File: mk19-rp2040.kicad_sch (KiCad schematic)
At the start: 134 parts, among them J1 USB_C_Receptacle_USB2.0, J10 Conn_01x02, J11 Conn_01x03_Socket, J12 USB_C_Receptacle_USB2.0, J13 USB_C_Receptacle_USB2.0, J3 Conn_01x02_Socket, J5 Conn_01x02, J7 Conn_01x02_Socket, J8 Conn_01x02_Socket, J9 Conn_01x02_Socket, T1 Conn_01x01_Socket, T10 Conn_01x01_Socket, T11 Conn_01x01_Socket, T12 Conn_01x01_Socket, T13 Conn_01x01_Socket, T14 Conn_01x01_Socket, T15 Conn_01x01_Socket, T2 Conn_01x01_Socket, T3 Conn_01x01_Socket, T5 Conn_01x01_Socket, T6 Conn_01x01_Socket, T7 Conn_01x01_Socket, T8 Conn_01x01_Socket, T9 Conn_01x01_Socket, U1 RP2040, U10 1N4148W_C81598, U11 1N4148W_C81598, U12 1N4148W_C81598, U13 1N4148W_C81598, U14 1N4148W_C81598, U15 1N4148W_C81598, U2 USBLC6-2P6, U3 XC6210B332MR-G, U4 USBLC6-2P6, U5 W25Q128JVS, U6 8_01A0_008200, U7 8_01A0_008200, U8 USBLC6-2P6, U9 1N4148W_C81598, Y1 Crystal_GND24

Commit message: some bad footprints, other fixes
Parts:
- 5WAY1, FAL1, FAL2, PWM1: footprint Connector_JST:JST_XH_B3B-XH-AM_1x08_P2.50mm_Horizontal -> Connector_JST:JST_XH_S8B-XH-A_1x08_P2.50mm_Horizontal
- COL1, COL2, ROW1, ROW2: footprint Connector_JST:JST_EH_S8B-EH_1x08_P2.50mm_Horizontal -> Connector_JST:JST_XH_S8B-XH-A_1x08_P2.50mm_Horizontal
- J1, J12, J13: footprint drawings:GT-USB-7014C -> ct-kicad:USB-C-SMD_12P-P0.50-H-F_TYPE-C-31-M-14
- J3, J7, J8, J9, PWR-EXT-IN1: footprint Connector_JST:JST_XH_B3B-XH-AM_1x02_P2.50mm_Vertical -> Connector_JST:JST_XH_B2B-XH-AM_1x02_P2.50mm_Vertical
- VANILED1: footprint Connector_JST:JST_XH_B3B-XH-AM_1x08_P2.50mm_Vertical -> Connector_JST:JST_XH_B8B-XH-AM_1x08_P2.50mm_Vertical
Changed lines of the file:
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@@
 			)
 		)
-		(property "Footprint" "Connector_JST:JST_XH_B3B-XH-AM_1x08_P2.50mm_Horizontal"
+		(property "Footprint" "Connector_JST:JST_XH_S8B-XH-A_1x08_P2.50mm_Horizontal"
 			(at 158.75 271.78 0)
 			(effects
@@
 			)
 		)
-		(property "Footprint" "Connector_JST:JST_XH_B3B-XH-AM_1x08_P2.50mm_Horizontal"
+		(property "Footprint" "Connector_JST:JST_XH_S8B-XH-A_1x08_P2.50mm_Horizontal"
 			(at 100.33 269.24 0)
 			(effects
@@
 			)
 		)
-		(property "Footprint" "drawings:GT-USB-7014C"
+		(property "Footprint" "ct-kicad:USB-C-SMD_12P-P0.50-H-F_TYPE-C-31-M-14"
 			(at 373.38 367.03 0)
 			(effects
@@
 			)
 		)
-		(property "Footprint" "Connector_JST:JST_XH_B3B-XH-AM_1x02_P2.50mm_Vertical"
+		(property "Footprint" "Connector_JST:JST_XH_B2B-XH-AM_1x02_P2.50mm_Vertical"
 			(at 229.87 429.26 0)
 			(effects
@@
 			)
 		)
-		(property "Footprint" "Connector_JST:JST_XH_B3B-XH-AM_1x02_P2.50mm_Vertical"
+		(property "Footprint" "Connector_JST:JST_XH_B2B-XH-AM_1x02_P2.50mm_Vertical"
 			(at 134.62 411.48 0)
 			(effects
@@
 			)
 		)
-		(property "Footprint" "Connector_JST:JST_XH_B3B-XH-AM_1x08_P2.50mm_Horizontal"
+		(property "Footprint" "Connector_JST:JST_XH_S8B-XH-A_1x08_P2.50mm_Horizontal"
 			(at 46.99 269.24 0)
 			(effects
@@
 			)
 		)
-		(property "Footprint" "drawings:GT-USB-7014C"
+		(property "Footprint" "ct-kicad:USB-C-SMD_12P-P0.50-H-F_TYPE-C-31-M-14"
 			(at 374.65 237.49 0)
 			(effects
@@
 			)
 		)
-		(property "Footprint" "Connector_JST:JST_EH_S8B-EH_1x08_P2.50mm_Horizontal"
+		(property "Footprint" "Connector_JST:JST_XH_S8B-XH-A_1x08_P2.50mm_Horizontal"
 			(at 44.45 148.59 0)
 			(effects
@@
 			)
 		)
-		(property "Footprint" "Connector_JST:JST_EH_S8B-EH_1x08_P2.50mm_Horizontal"
+		(property "Footprint" "Connector_JST:JST_XH_S8B-XH-A_1x08_P2.50mm_Horizontal"
 			(at 71.12 148.59 0)
 			(effects
@@
 			)
 		)
-		(property "Footprint" "Connector_JST:JST_XH_B3B-XH-AM_1x02_P2.50mm_Vertical"
+		(property "Footprint" "Connector_JST:JST_XH_B2B-XH-AM_1x02_P2.50mm_Vertical"
 			(at 209.55 403.86 0)
 			(effects
@@
 			)
 		)
-		(property "Footprint" "Connector_JST:JST_EH_S8B-EH_1x08_P2.50mm_Horizontal"
+		(property "Footprint" "Connector_JST:JST_XH_S8B-XH-A_1x08_P2.50mm_Horizontal"
 			(at 71.12 123.19 0)
 			(effects
@@
 			)
 		)
-		(property "Footprint" "Connector_JST:JST_XH_B3B-XH-AM_1x08_P2.50mm_Vertical"
+		(property "Footprint" "Connector_JST:JST_XH_B8B-XH-AM_1x08_P2.50mm_Vertical"
 			(at 166.37 370.84 0)
 			(effects
@@
 			)
 		)
-		(property "Footprint" "drawings:GT-USB-7014C"
+		(property "Footprint" "ct-kicad:USB-C-SMD_12P-P0.50-H-F_TYPE-C-31-M-14"
 			(at 373.38 302.26 0)
 			(effects
@@
 			)
 		)
-		(property "Footprint" "Connector_JST:JST_XH_B3B-XH-AM_1x02_P2.50mm_Vertical"
+		(property "Footprint" "Connector_JST:JST_XH_B2B-XH-AM_1x02_P2.50mm_Vertical"
 			(at 118.11 331.47 0)
 			(effects
@@
 			)
 		)
-		(property "Footprint" "Connector_JST:JST_EH_S8B-EH_1x08_P2.50mm_Horizontal"
+		(property "Footprint" "Connector_JST:JST_XH_S8B-XH-A_1x08_P2.50mm_Horizontal"
 			(at 44.45 123.19 0)
 			(effects
@@
 			)
 		)
-		(property "Footprint" "Connector_JST:JST_XH_B3B-XH-AM_1x02_P2.50mm_Vertical"
+		(property "Footprint" "Connector_JST:JST_XH_B2B-XH-AM_1x02_P2.50mm_Vertical"
 			(at 248.92 403.86 0)
 			(effects
@@
 			)
 		)
-		(property "Footprint" "Connector_JST:JST_XH_B3B-XH-AM_1x08_P2.50mm_Horizontal"
+		(property "Footprint" "Connector_JST:JST_XH_S8B-XH-A_1x08_P2.50mm_Horizontal"
 			(at 203.2 271.78 0)
 			(effects

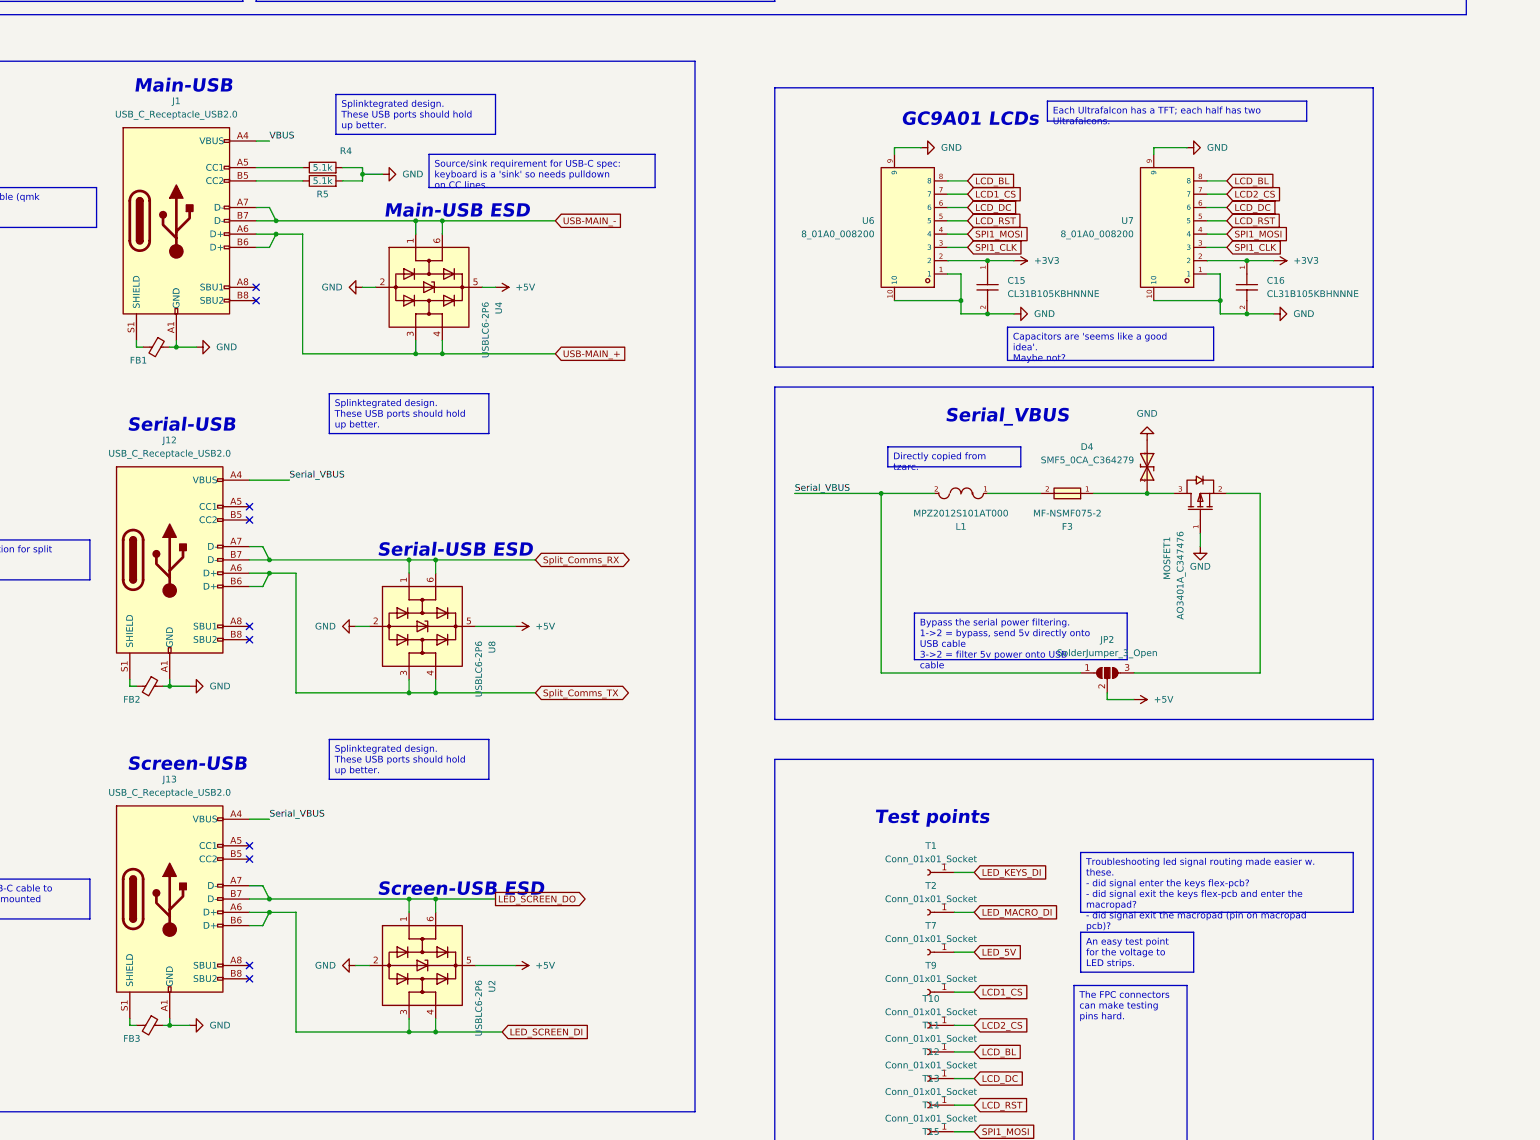
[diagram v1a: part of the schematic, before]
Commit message: progress update
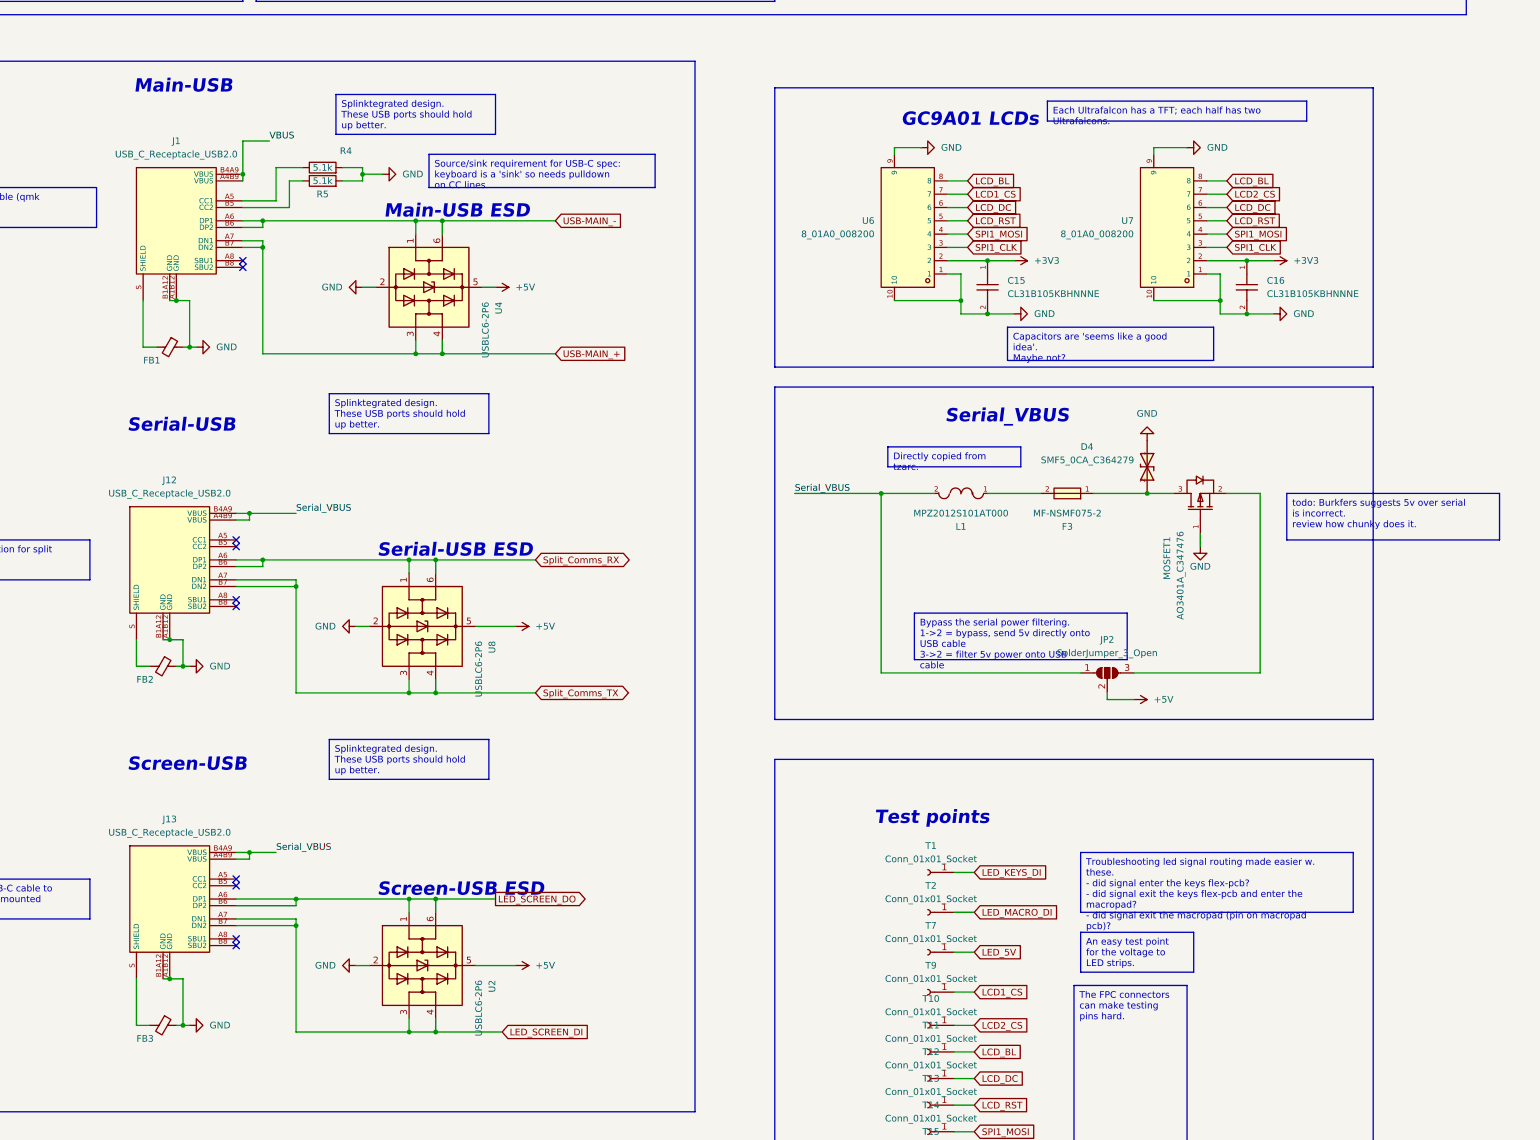
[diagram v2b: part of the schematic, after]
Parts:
- J1, J12, J13: symbol Connector:USB_C_Receptacle_USB2.0 -> ct-kicad:TYPE-C-31-M-14
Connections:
- net GND: now also J1.A1B12 (GND), J1.B1A12 (GND), J12.A1B12 (GND), J12.B1A12 (GND), J13.A1B12 (GND), J13.B1A12 (GND); no longer J1.A1 (GND), J1.A12 (GND), J1.B1 (GND), J1.B12 (GND), J12.A1 (GND), J12.A12 (GND), J12.B1 (GND), J12.B12 (GND), J13.A1 (GND), J13.A12 (GND), J13.B1 (GND), J13.B12 (GND)
- net LED_SCREEN_DI: now also J13.A7 (DN1), J13.B7 (DN2); no longer J13.A6 (D+), J13.B6 (D+)
- net LED_SCREEN_DO: now also J13.A6 (DP1), J13.B6 (DP2); no longer J13.A7 (D-), J13.B7 (D-)
- net Serial_VBUS: now also J12.A4B9 (VBUS), J12.B4A9 (VBUS), J13.A4B9 (VBUS), J13.B4A9 (VBUS); no longer J12.A4 (VBUS), J12.A9 (VBUS), J12.B4 (VBUS), J12.B9 (VBUS), J13.A4 (VBUS), J13.A9 (VBUS), J13.B4 (VBUS), J13.B9 (VBUS)
- net Split_Comms_RX: now also J12.A6 (DP1), J12.B6 (DP2); no longer J12.A7 (D-), J12.B7 (D-)
- net Split_Comms_TX: now also J12.A7 (DN1), J12.B7 (DN2); no longer J12.A6 (D+), J12.B6 (D+)
- net USB-MAIN_+: now also J1.A7 (DN1), J1.B7 (DN2); no longer J1.A6 (D+), J1.B6 (D+)
- net USB-MAIN_-: now also J1.A6 (DP1), J1.B6 (DP2); no longer J1.A7 (D-), J1.B7 (D-)
- net VBUS: now also J1.A4B9 (VBUS), J1.B4A9 (VBUS); no longer J1.A4 (VBUS), J1.A9 (VBUS), J1.B4 (VBUS), J1.B9 (VBUS)
- net at FB3.2: now also J13.S (SHIELD); no longer J13.S1 (SHIELD)
- net at FB2.2: now also J12.S (SHIELD); no longer J12.S1 (SHIELD)
- net at FB1.2: now also J1.S (SHIELD); no longer J1.S1 (SHIELD)
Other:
- moved on the sheet: FB1, FB2, FB3
